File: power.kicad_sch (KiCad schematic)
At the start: 41 parts, among them IC1 LM2678SD-5.0_NOPB, J12 USB_C_Receptacle_USB2.0_14P, Q1 2N7000, Q20 NPN, Q21 NPN, U1 UA78M33QDCYRQ1, U2 SFH617A-1, U4 CP2102N-Axx-xQFN28

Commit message: Update power.kicad_sch
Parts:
- removed D2, D3: D, Diode_THT:D_A-405_P7.62mm_Horizontal, symbol Device:D
- removed Q1: 2N7000, Package_TO_SOT_THT:TO-92_Inline, symbol Transistor_FET:2N7000
- removed R1: 470, Resistor_THT:R_Axial_DIN0207_L6.3mm_D2.5mm_P10.16mm_Horizontal, symbol Device:R
- removed U2: SFH617A-1, Package_DIP:DIP-4_W7.62mm, symbol Isolator:SFH617A-1
- added C10: 100n, symbol Device:C
- added D10, D11: D_Zener, symbol Device:D_Zener
- added D8, D9: D, Diode_THT:D_A-405_P7.62mm_Horizontal, symbol Device:D
- added Q2: NMOS, symbol Simulation_SPICE:NMOS
- added Q3: PMOS, symbol Simulation_SPICE:PMOS
- added R2: 1k, Resistor_THT:R_Axial_DIN0207_L6.3mm_D2.5mm_P10.16mm_Horizontal, symbol Device:R
- added R3, R5: 100k, symbol Device:R
- added R4, R6, R7: 10k, symbol Device:R
- added U3: SFH617A-1, Package_DIP:DIP-4_W7.62mm, symbol Isolator:SFH617A-1
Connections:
- net +3.3V: now also U3.4
- net Constant Power: now also C10.1, D10.1 (K), Q3.3 (S), R3.1
- net GND: now also D11.2 (A), Q2.3 (S), R2.2, R5.2, R7.1
- net Ignition_Sensor: now also R7.2, U3.3
- net Power_Off: now also D9.2 (A)
- net Switched Power: now also U3.1
- net VAA: now also Q3.1 (D)
- new net: C10.2, D10.2 (A), Q3.2 (G), R3.2, R4.1
- new net: Q2.1 (D), R4.2
- new net: D11.1 (K), Q2.2 (G), R5.1, R6.1
- new net: D8.1 (K), D9.1 (K), R6.2
- new net: D8.2 (A), R2.1, U3.2
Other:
- moved on the sheet: C13, C14, C15, D19, D20, D4, D5, D6, D7, F2, J12, Q20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

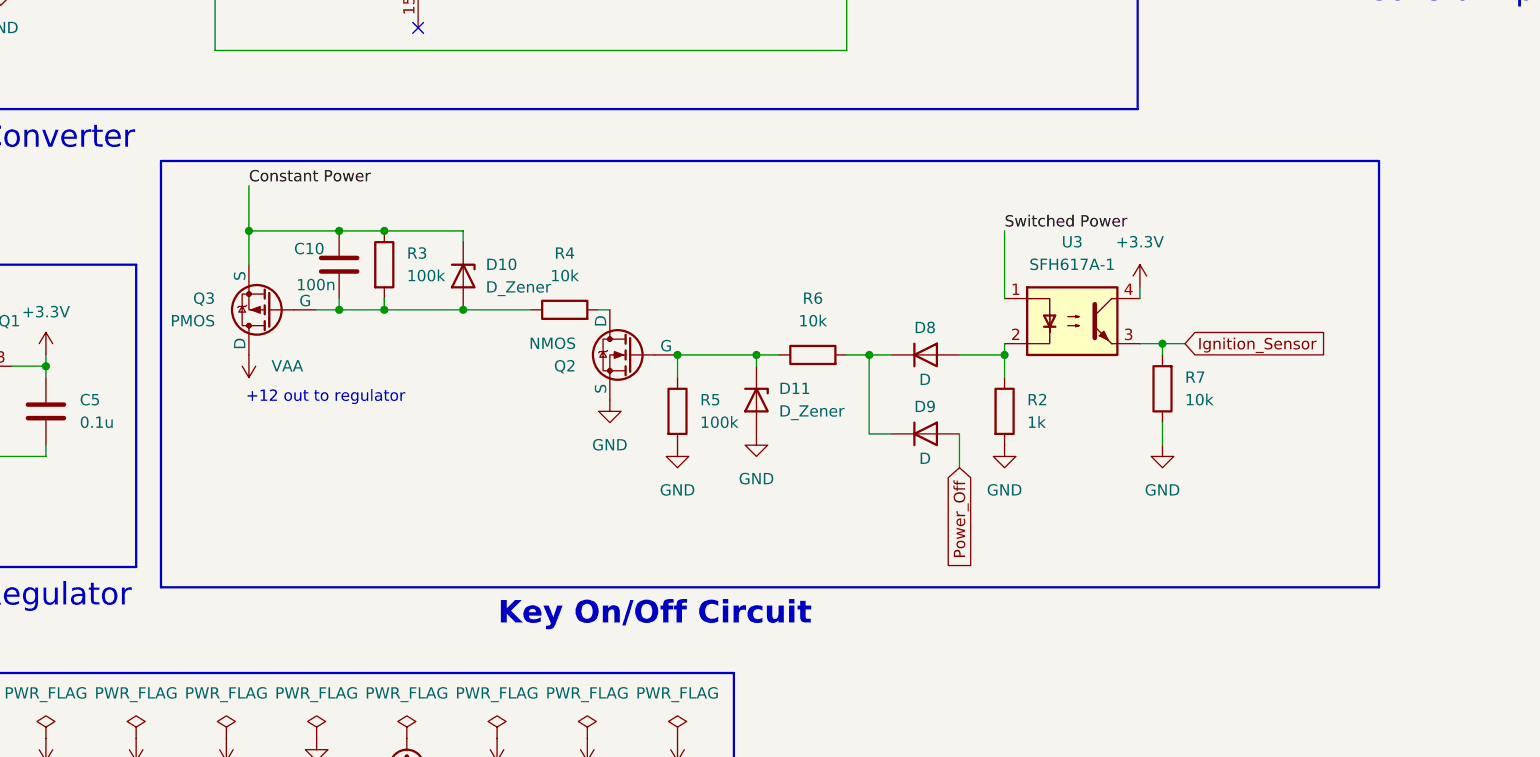
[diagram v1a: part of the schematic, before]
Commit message: update
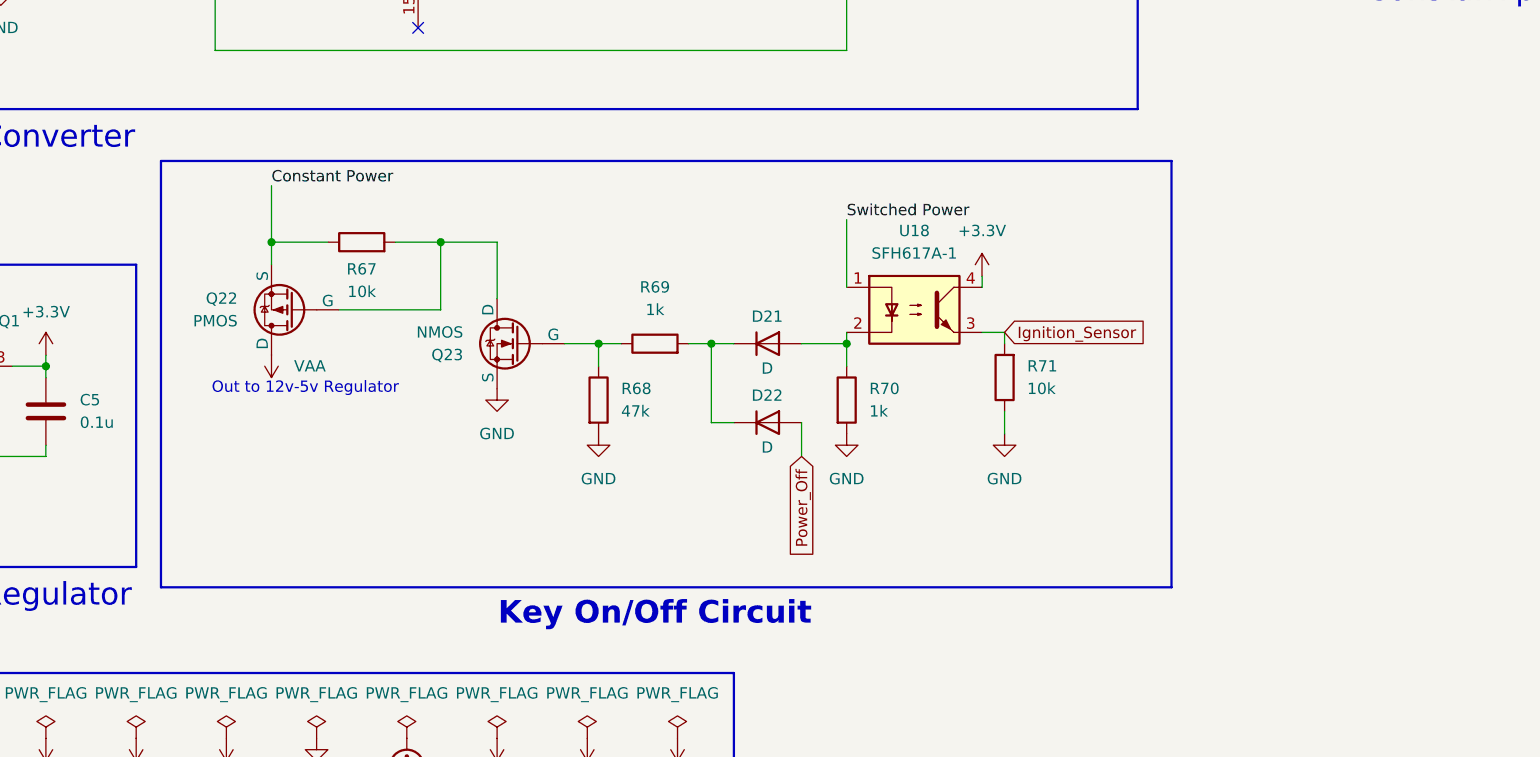
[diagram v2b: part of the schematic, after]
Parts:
- removed C10: 100n, symbol Device:C
- removed D10, D11: D_Zener, symbol Device:D_Zener
- removed D8, D9: D, Diode_THT:D_A-405_P7.62mm_Horizontal, symbol Device:D
- removed Q2: NMOS, symbol Simulation_SPICE:NMOS
- removed Q3: PMOS, symbol Simulation_SPICE:PMOS
- removed R2: 1k, Resistor_THT:R_Axial_DIN0207_L6.3mm_D2.5mm_P10.16mm_Horizontal, symbol Device:R
- removed R3, R5: 100k, symbol Device:R
- removed R4, R6, R7: 10k, symbol Device:R
- removed U3: SFH617A-1, Package_DIP:DIP-4_W7.62mm, symbol Isolator:SFH617A-1
- added D21, D22: D, Diode_THT:D_A-405_P7.62mm_Horizontal, symbol Device:D
- added Q22: PMOS, Package_TO_SOT_THT:TO-220-3_Vertical, symbol Simulation_SPICE:PMOS
- added Q23: NMOS, Package_TO_SOT_THT:TO-220-3_Vertical, symbol Simulation_SPICE:NMOS
- added R67, R71: 10k, Resistor_THT:R_Axial_DIN0207_L6.3mm_D2.5mm_P10.16mm_Horizontal, symbol Device:R
- added R68: 47k, Resistor_THT:R_Axial_DIN0207_L6.3mm_D2.5mm_P10.16mm_Horizontal, symbol Device:R
- added R69, R70: 1k, Resistor_THT:R_Axial_DIN0207_L6.3mm_D2.5mm_P10.16mm_Horizontal, symbol Device:R
- added U18: SFH617A-1, Package_DIP:DIP-4_W7.62mm, symbol Isolator:SFH617A-1
- L1: footprint Inductor_THT:L_Radial_D9.5mm_P5.00mm_Fastron_07HVP -> Inductor_THT:L_Axial_L9.5mm_D4.0mm_P15.24mm_Horizontal_Fastron_SMCC
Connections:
- net +3.3V: now also U18.4
- net Constant Power: now also Q22.3 (S), R67.1
- net GND: now also Q23.3 (S), R68.2, R70.2, R71.1
- net Ignition_Sensor: now also R71.2, U18.3
- net Power_Off: now also D22.2 (A)
- net Switched Power: now also U18.1
- net VAA: now also Q22.1 (D)
- new net: Q23.2 (G), R68.1, R69.1
- new net: D21.1 (K), D22.1 (K), R69.2
- new net: Q22.2 (G), Q23.1 (D), R67.2
- new net: D21.2 (A), R70.1, U18.2
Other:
- note added: "Out to 12v-5v Regulator"
- note removed: "+12 out to regulator"
